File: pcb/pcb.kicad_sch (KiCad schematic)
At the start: 52 parts

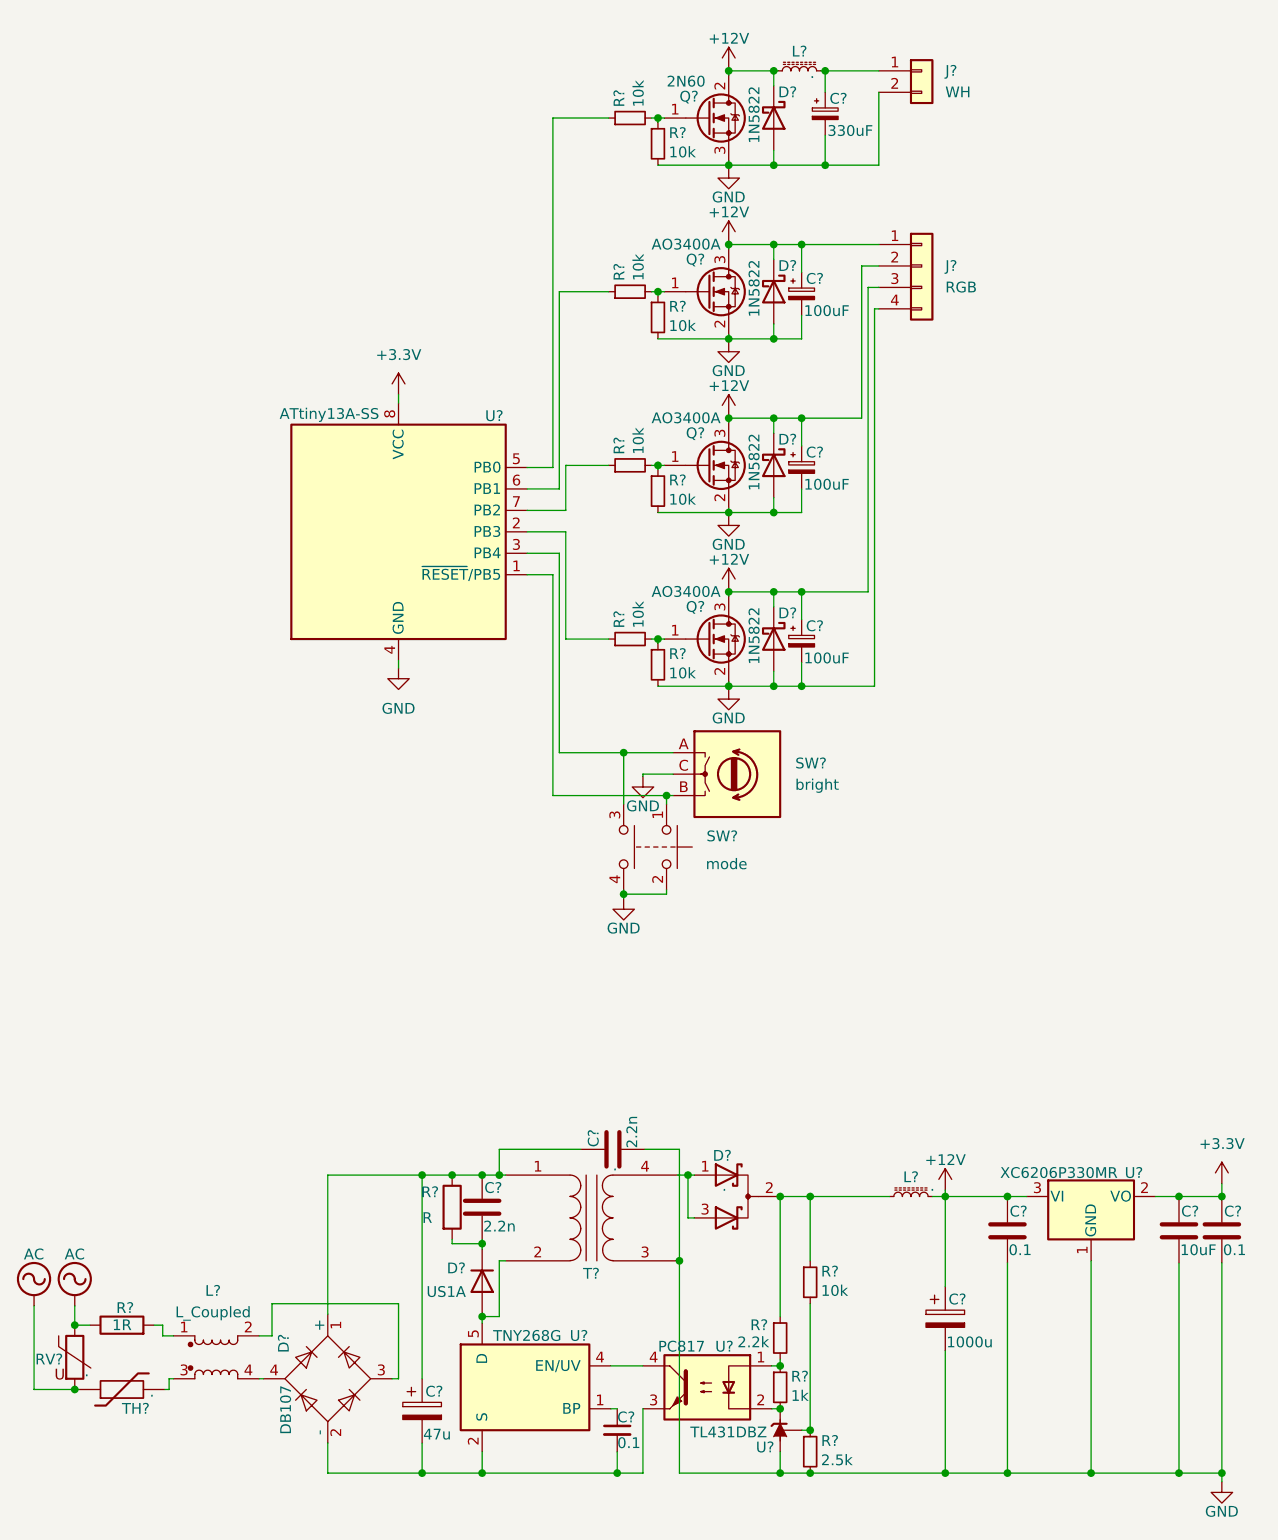
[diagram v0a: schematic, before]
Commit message: err in sch
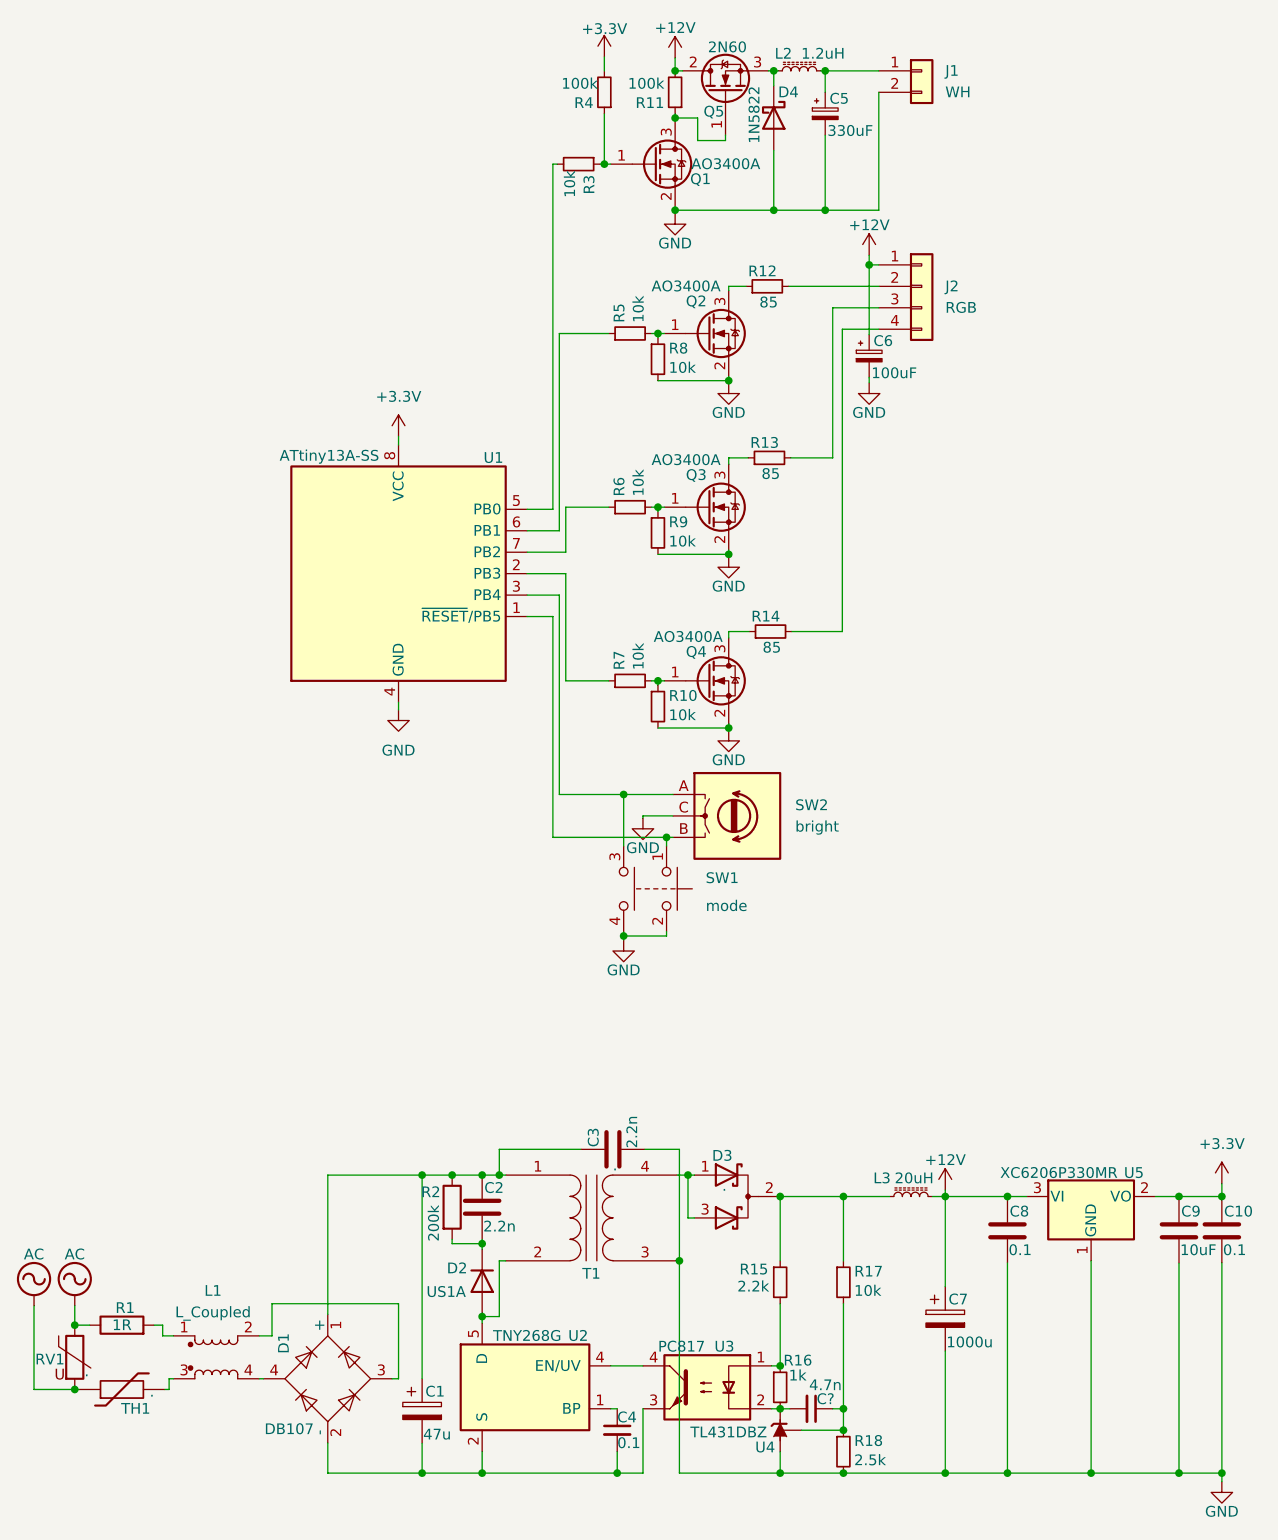
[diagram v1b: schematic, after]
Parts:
- removed C? (x2): 100uF, symbol Device:C_Polarized_Small
- removed D? (x3): 1N5822, Diode_THT:D_DO-201AD_P15.24mm_Horizontal, symbol Diode:1N5822
- removed R? (x2): 10k, symbol Device:R_Small
- added C?: 4.7n, symbol Device:C_Small
- added Q1: AO3400A, Package_TO_SOT_SMD:SOT-23, symbol Transistor_FET:AO3400A
- added R11, R4: 100k, symbol Device:R_Small
- added R12, R13, R14: 85, symbol Device:R_Small
- added R3: 10k, symbol Device:R_Small
- L2: renamed from L?; value . -> 1.2uH
- L3: renamed from L?; value . -> 20uH
- R2: renamed from R?; value R -> 200k
- gave numbers to parts that had none: 42
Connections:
- net +12V: now also R11.2; no longer D4.1 (K), J2.2 (Pin_2), J2.3 (Pin_3), L2.1, Q2.3 (D), Q3.3 (D), Q4.3 (D)
- net +3V3: now also R4.2
- net GND: now also Q1.2 (S); no longer J2.4 (Pin_4), Q5.3 (S)
- net at U1.5 (PB0): now also R3.2
- net at Q5.1 (G): now also Q1.3 (D), R11.1
- net at R17.2, R18.1, U4.2 (REF): now also C?.1
- net at R16.2, U3.2, U4.1 (K): now also C?.2
- new net: Q3.3 (D), R13.1
- new net: J2.3 (Pin_3), R13.2
- new net: J2.2 (Pin_2), R12.2
- new net: J2.4 (Pin_4), R14.2
- new net: D4.1 (K), L2.1, Q5.3 (S)
- new net: Q2.3 (D), R12.1
- new net: Q4.3 (D), R14.1
- new net: Q1.1 (G), R3.1, R4.1
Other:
- moved on the sheet: C6, J2, Q2, Q3, Q4, Q5, R10, R15, R17, R18, R5, R6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
